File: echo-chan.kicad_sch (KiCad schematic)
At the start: 50 parts, among them J1 SJ1-3533NS, J2 USB_B, SW1 SW_Push, T1 Transformer_1P_1S, U1 JAMMA, U2 JAMMA, U3 AT90USB1286, U4 HD15, U6 THS7374, Y1 16MHz

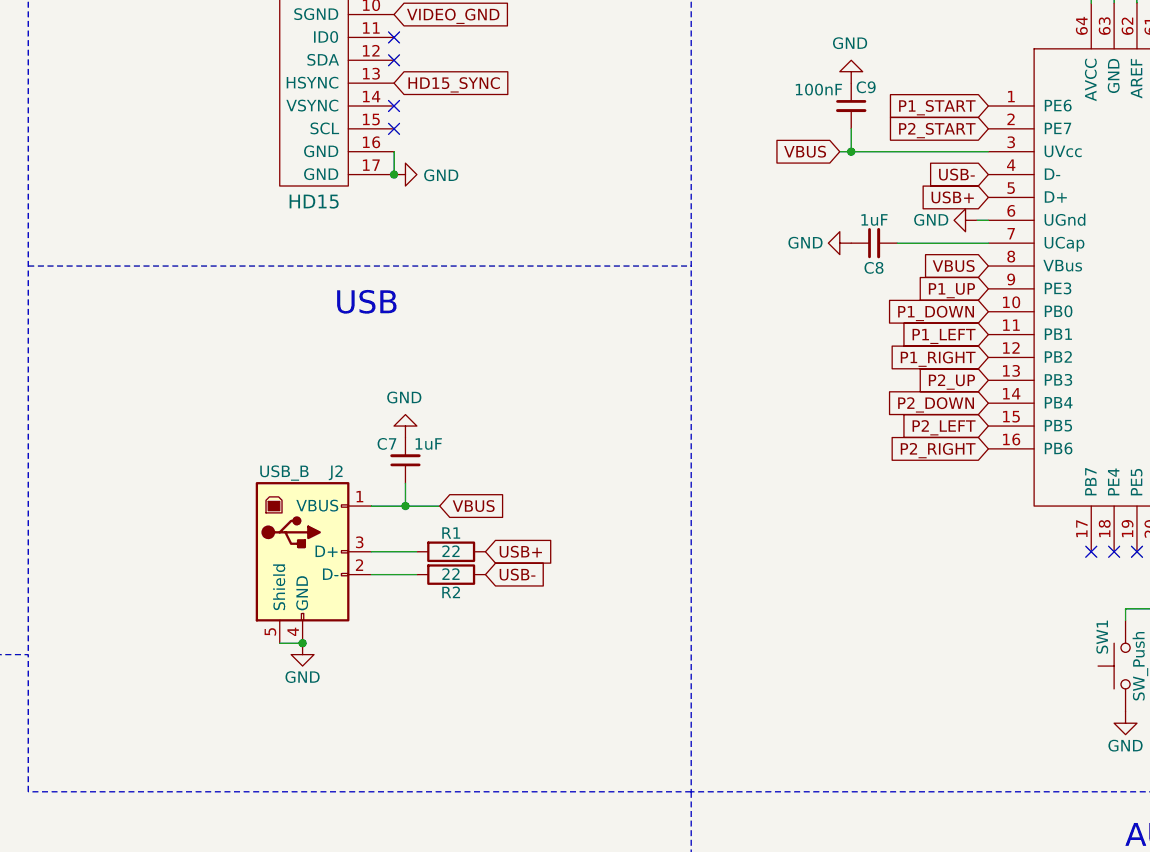
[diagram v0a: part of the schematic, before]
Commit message: checkpoint
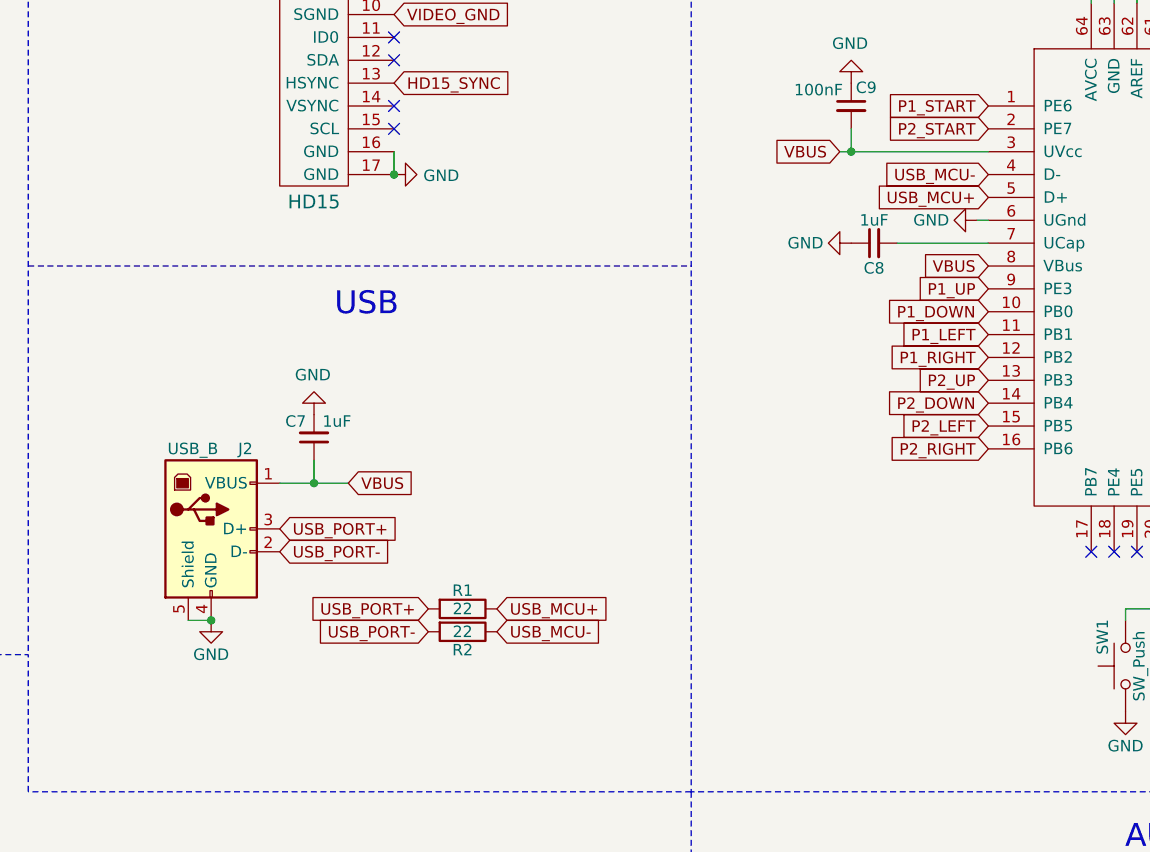
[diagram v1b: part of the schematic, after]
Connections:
- net USB_PORT+: now reaches J2.3 (D+), R1.2
- net USB_PORT-: now reaches J2.2 (D-), R2.2
- net USB+ renamed USB_MCU+
- net USB- renamed USB_MCU-
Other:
- moved on the sheet: C7, J2, R1, R2
